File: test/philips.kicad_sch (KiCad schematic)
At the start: 79 parts, among them J2 Conn_01x02, Q1 BC859, Q10 BC848, Q11 BC808, Q12 BC848, Q14 BC808, Q2 BC859, Q3 BC859, Q4 BC859, Q5 BC859, Q6 BC848, Q7 BC808, Q8 BC848, Q9 BC808, U3 PCA9531PW, U4 PCF8574AT

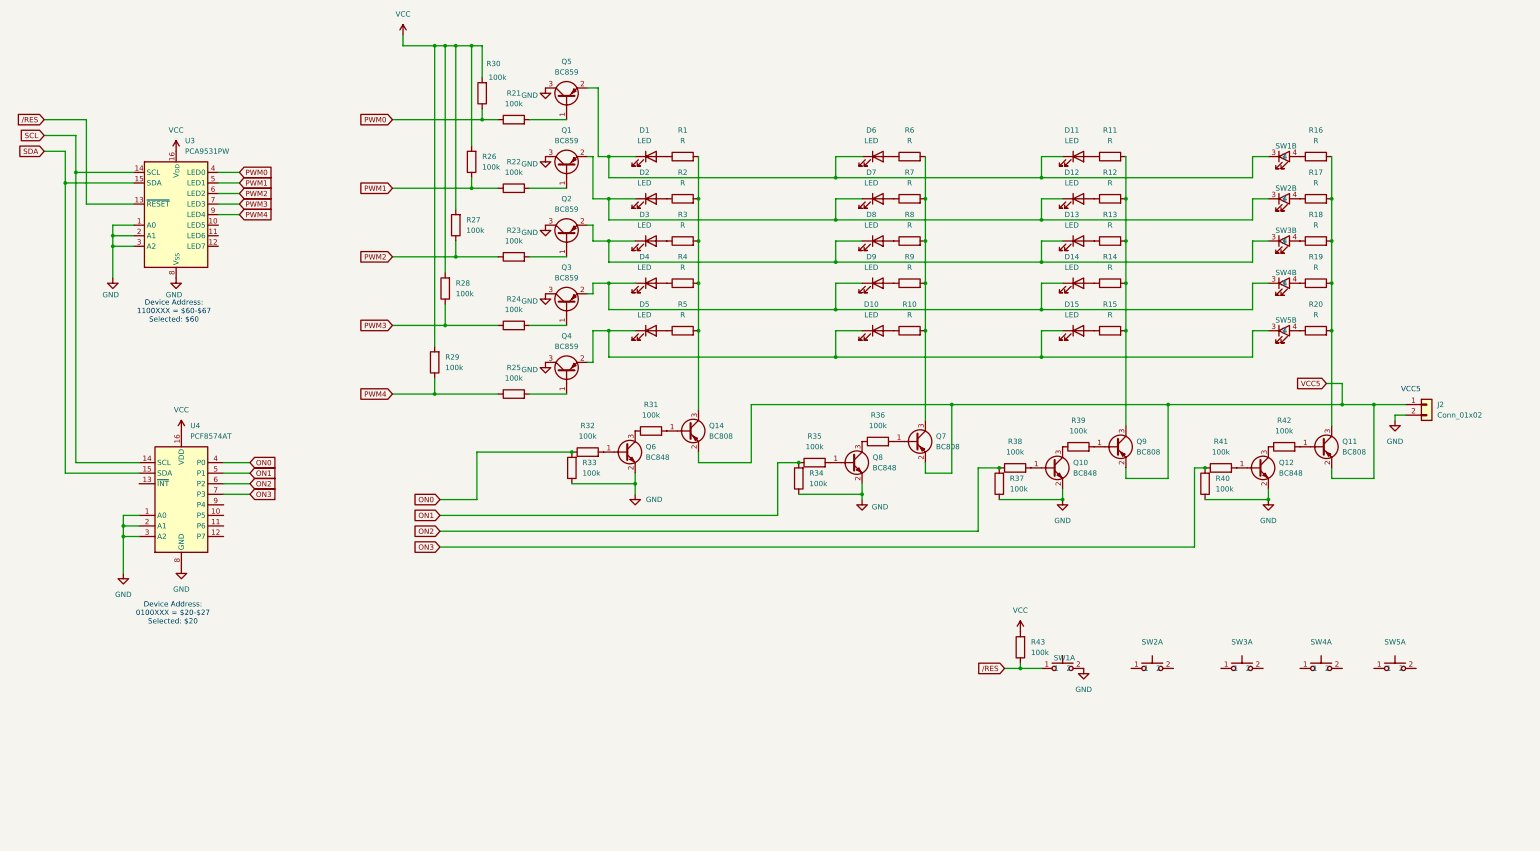
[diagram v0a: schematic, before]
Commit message: work on 2nd update test
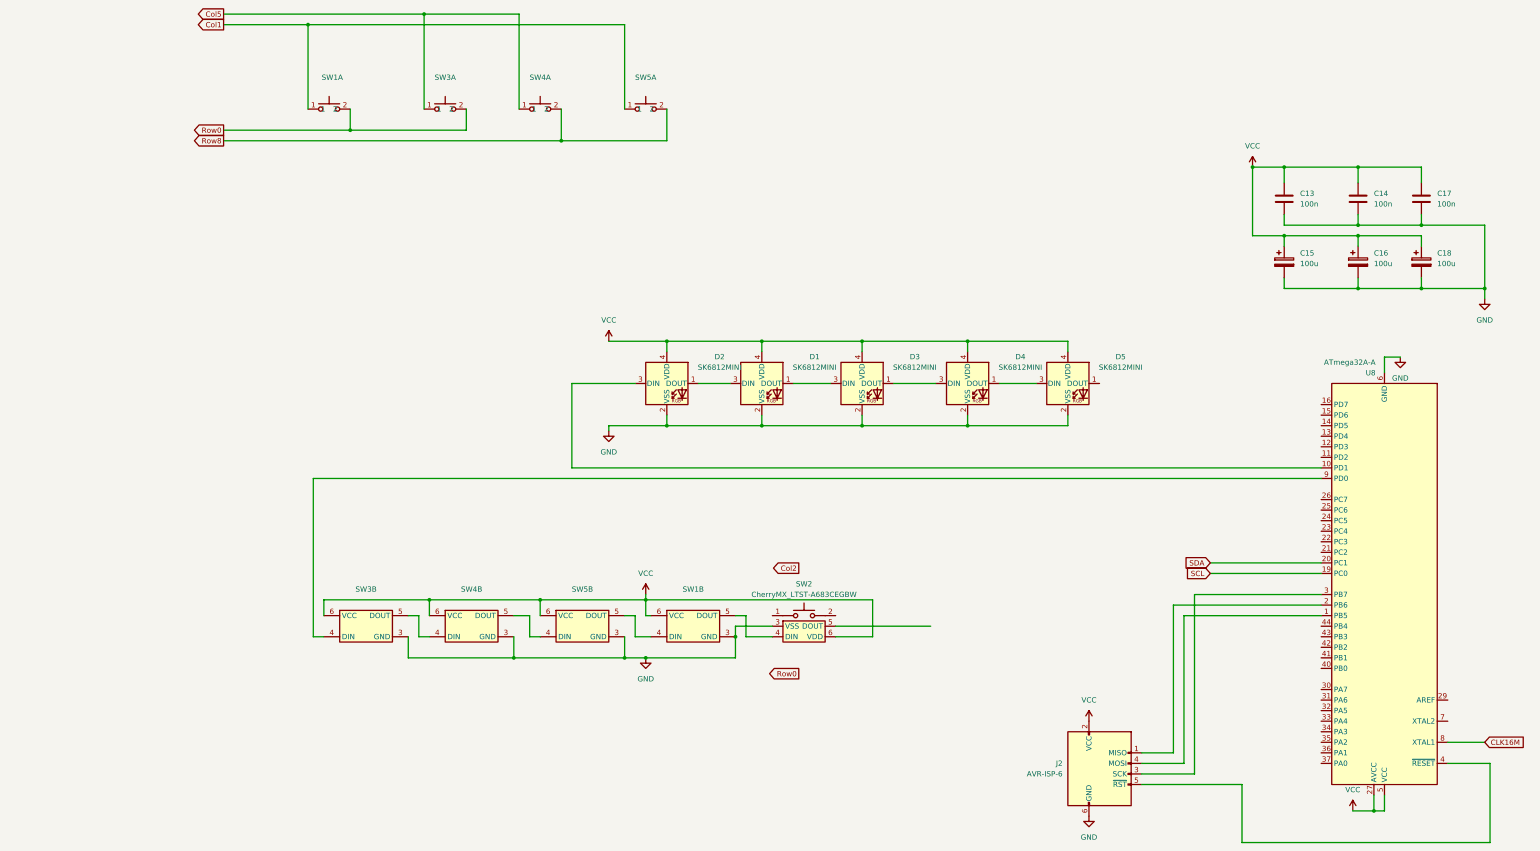
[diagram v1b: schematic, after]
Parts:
- removed D1, D10, D11, D12, D13, D14, D15, D2, D3, D4, D5, D6, D7, D8, D9: LED, LED_THT:LED_D3.0mm, symbol Device:LED
- removed J2: Conn_01x02, Connector_PinHeader_2.54mm:PinHeader_1x02_P2.54mm_Vertical, symbol Connector_Generic:Conn_01x02
- removed Q1, Q2, Q3, Q4, Q5: BC859, Package_TO_SOT_SMD:SOT-23, symbol Transistor_BJT:BC859
- removed Q10, Q12, Q6, Q8: BC848, Package_TO_SOT_SMD:SOT-23, symbol Transistor_BJT:BC848
- removed Q11, Q14, Q7, Q9: BC808, Package_TO_SOT_SMD:SOT-23, symbol Transistor_BJT:BC808
- removed R1, R10, R11, R12, R13, R14, R15, R16, R17, R18, R19, R2, R20, R3, R4, R5, R6, R7, R8, R9: R, Resistor_THT:R_Axial_DIN0204_L3.6mm_D1.6mm_P2.54mm_Vertical, symbol Device:R
- removed R21, R22, R23, R24, R25, R26, R27, R28, R29, R30, R31, R32, R33, R34, R35, R36, R37, R38, R39, R40, R41, R42, R43: 100k, Resistor_THT:R_Axial_DIN0204_L3.6mm_D1.6mm_P2.54mm_Vertical, symbol Device:R
- removed unit 2 of SW1
- removed SW2, SW3, SW4, SW5: ~, petkn:SW_Cherry_MX_1.00u_PCB_with_LED, symbol petkn:MX Key with LED Unit
- removed U3: PCA9531PW, Package_SO:TSSOP-16_4.4x5mm_P0.65mm, symbol Driver_LED:PCA9531PW
- removed U4: PCF8574AT, Package_SO:SOIC-16W_7.5x10.3mm_P1.27mm, symbol Interface_Expansion:PCF8574AT
- added C13, C14, C17: 100n, Capacitor_SMD:C_0805_2012Metric_Pad1.18x1.45mm_HandSolder, symbol Device:C
- added C15, C16, C18: 100u, Capacitor_SMD:C_1206_3216Metric_Pad1.33x1.80mm_HandSolder, symbol Device:C_Polarized
- added D1, D2, D3, D4, D5: SK6812MINI, LED_SMD:LED_SK6812MINI_PLCC4_3.5x3.5mm_P1.75mm, symbol LED:SK6812MINI
- added J2: AVR-ISP-6, Connector_IDC:IDC-Header_2x03_P2.54mm_Vertical, symbol Connector:AVR-ISP-6
- added unit 1 of SW1
- added SW2: CherryMX_LTST-A683CEGBW, petkn:SW_Cherry_MX_1.00u_PCB_with_RGB_LED, symbol CherryMX:CherryMX_LTST-A683CEGBW
- added SW3, SW4, SW5: ~, petkn:SW_Cherry_MX_1.00u_PCB_with_RGB_LED, symbol petkn:MX Key with SMD RGB LED
- added U8: ATmega32A-A, Package_QFP:TQFP-44_10x10mm_P0.8mm, symbol MCU_Microchip_ATmega:ATmega32A-A
- SW1: footprint petkn:SW_Cherry_MX_1.00u_PCB_with_LED -> CherryMX_PCB_LTST-A683CEGBW-Rotated:CherryMX_1.00u_PCB_LTST-A683CEGBW-Rotated; symbol petkn:MX Key with LED Unit -> petkn:MX Key with SMD RGB LED
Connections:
- net GND: now also SW1.3 (GND), C13.2, C14.2, C15.2, C16.2, C17.2, C18.2, D1.2 (VSS), D2.2 (VSS), D3.2 (VSS), D4.2 (VSS), D5.2 (VSS), J2.6 (GND), SW2.3 (VSS), SW3.3 (GND), SW4.3 (GND), SW5.3 (GND), U8.18 (GND), U8.28 (GND), U8.39 (GND), U8.6 (GND); no longer SW1.2
- net SCL: now also U8.19 (PC0)
- net SDA: now also U8.20 (PC1)
- net VCC: now also SW1.6 (VCC), C13.1, C14.1, C15.1, C16.1, C17.1, C18.1, D1.4 (VDD), D2.4 (VDD), D3.4 (VDD), D4.4 (VDD), D5.4 (VDD), J2.2 (VCC), SW2.6 (VDD), SW3.6 (VCC), SW4.6 (VCC), SW5.6 (VCC), U8.17 (VCC), U8.27 (AVCC), U8.38 (VCC), U8.5 (VCC)
- removed net /RES: SW1.1
- new net: D1.3 (DIN), D2.1 (DOUT)
- new net: D2.3 (DIN), U8.10 (PD1)
- new net: SW1.4 (DIN), SW5.5 (DOUT)
- new net: SW1.5 (DOUT), SW2.4 (DIN)
- new net: D4.1 (DOUT), D5.3 (DIN)
- new net: D3.1 (DOUT), D4.3 (DIN)
- new net: D1.1 (DOUT), D3.3 (DIN)
- new net: J2.1 (MISO), U8.2 (PB6)
- new net: J2.3 (SCK), U8.3 (PB7)
- new net: J2.4 (MOSI), U8.1 (PB5)
- new net: J2.5 (~{RST}), U8.4 (~{RESET})
- new net: SW4.5 (DOUT), SW5.4 (DIN)
- new net: SW3.4 (DIN), U8.9 (PD0)
- new net: SW3.5 (DOUT), SW4.4 (DIN)
- new net CLK16M: U8.8 (XTAL1)
- new net Col1: SW1.1, SW5.1
- new net Col5: SW3.1, SW4.1
- new net Row0: SW1.2, SW3.2
- new net Row8: SW4.2, SW5.2
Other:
- note removed: "Device Address: 0100XXX = $20-$27 Selected: $20"
- note removed: "Device Address: 1100XXX = $60-$67 Selected: $60"
- note removed: "VCC5"
